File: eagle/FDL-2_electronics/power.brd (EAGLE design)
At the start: 46.7 x 34.3 mm, 6 parts, among them X1 Power, X2 Motor

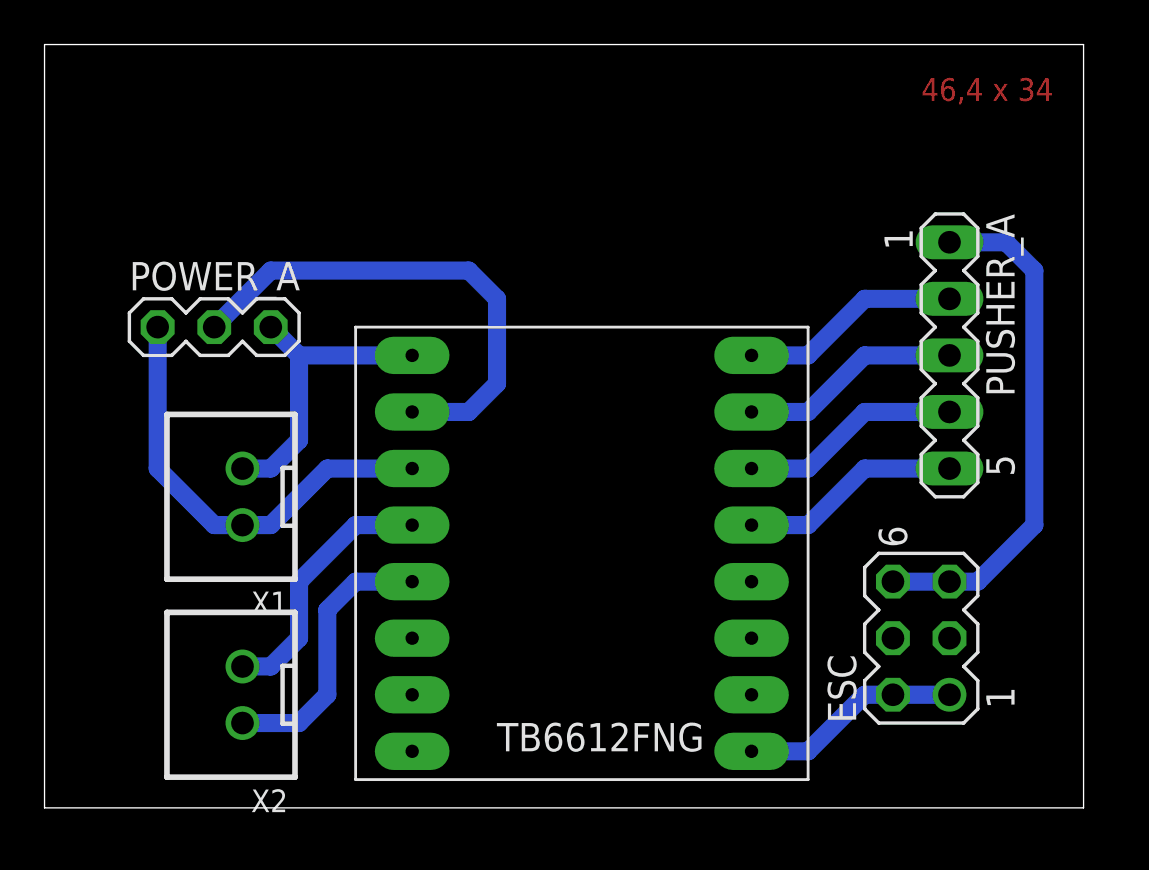
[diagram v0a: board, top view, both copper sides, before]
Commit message: some further work - mainly on pusher
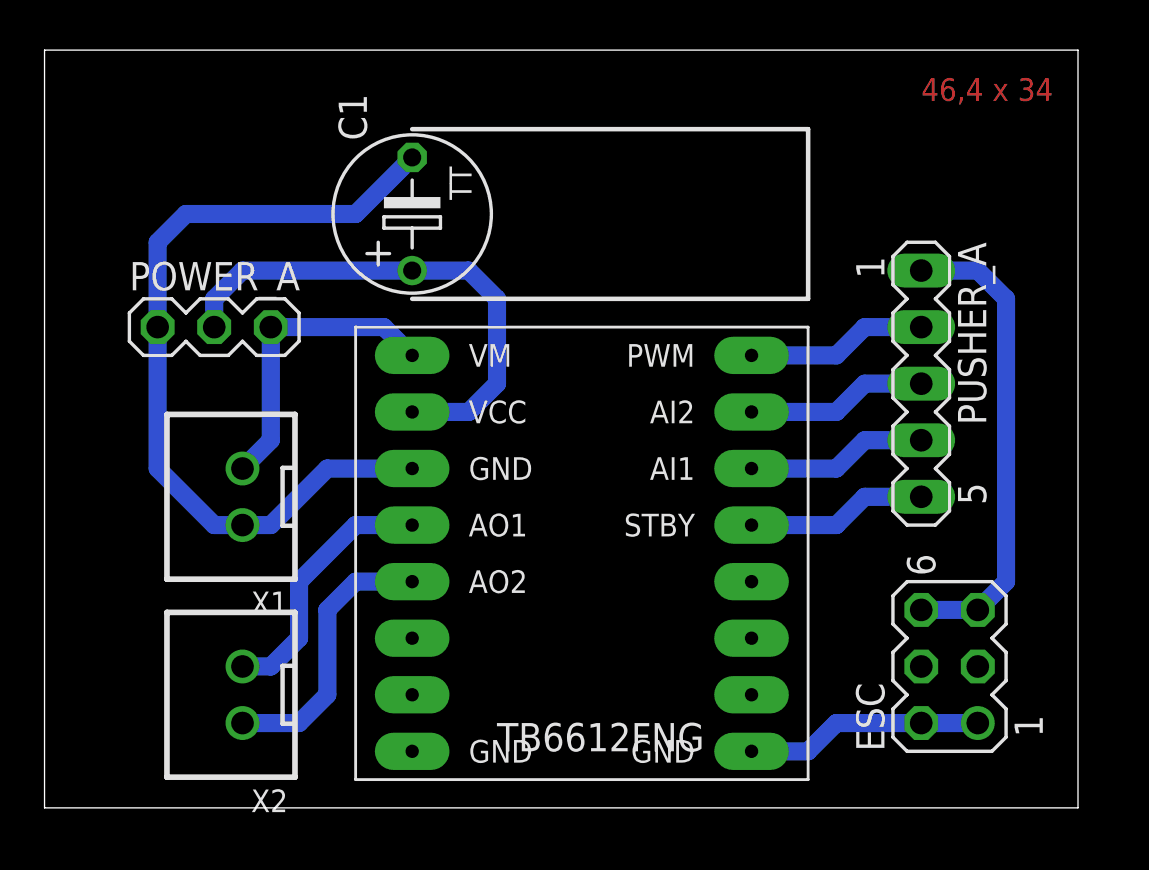
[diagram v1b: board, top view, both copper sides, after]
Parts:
- added C1: (no value), resistor:TT5D7
- moved ESC 1.80 mm to (40.6, 6.35)
- moved PUSHER_A 1.80 mm to (39.4, 19.1)
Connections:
- net N$28: now also C1.+
- net N$5: now also C1.-
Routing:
- net N$5: track 19.9 -> 36.7 mm
- net N$9: track 9.94 -> 8.15 mm
- net N$8: track 9.94 -> 8.15 mm
- net N$6: track 9.94 -> 8.15 mm
- net N$3: track 9.94 -> 8.15 mm
- net N$25: track 23.2 -> 21.4 mm
- net N$28: track 22.4 -> 23.2 mm
- net N$24: track 9.94 -> 10.7 mm
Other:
- board size 46.7 x 34.3 mm -> 46.4 x 34 mm
- board text added: "AI1"
- board text added: "AI2"
- board text added: "AO1"
- board text added: "AO2"
- board text added: "GND"
- board text added: "PWM"
- board text added: "STBY"
- board text added: "VCC"
- board text added: "VM"
